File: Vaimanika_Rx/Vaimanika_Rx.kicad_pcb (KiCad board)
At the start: 4 copper layers, 18 x 25 mm, 54 parts, among them T1 0900PC16J0042001E, U1 LR1121IMLTRT, U2 RFX2401C, U3 SKY13373-460LF, U4 ESP32-C3FH4, U5 TLV75533PDQNR, U6 OW2EL89CENUXFMYLC-32M, U7 ANT3216LL00R2400A, U8 TS2306A 240GF MSM 9_C2976675, X1 CJ17-400001010B20

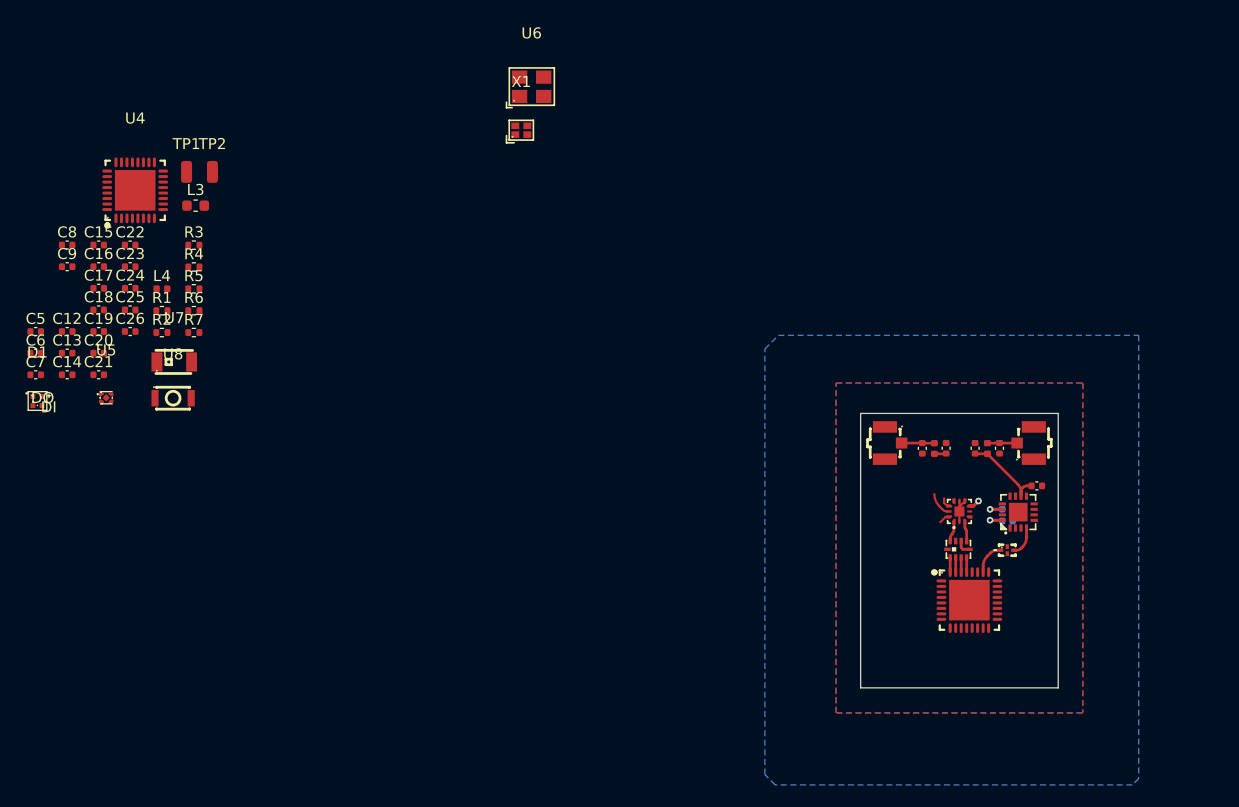
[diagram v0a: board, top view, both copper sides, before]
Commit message: 27-05-2026
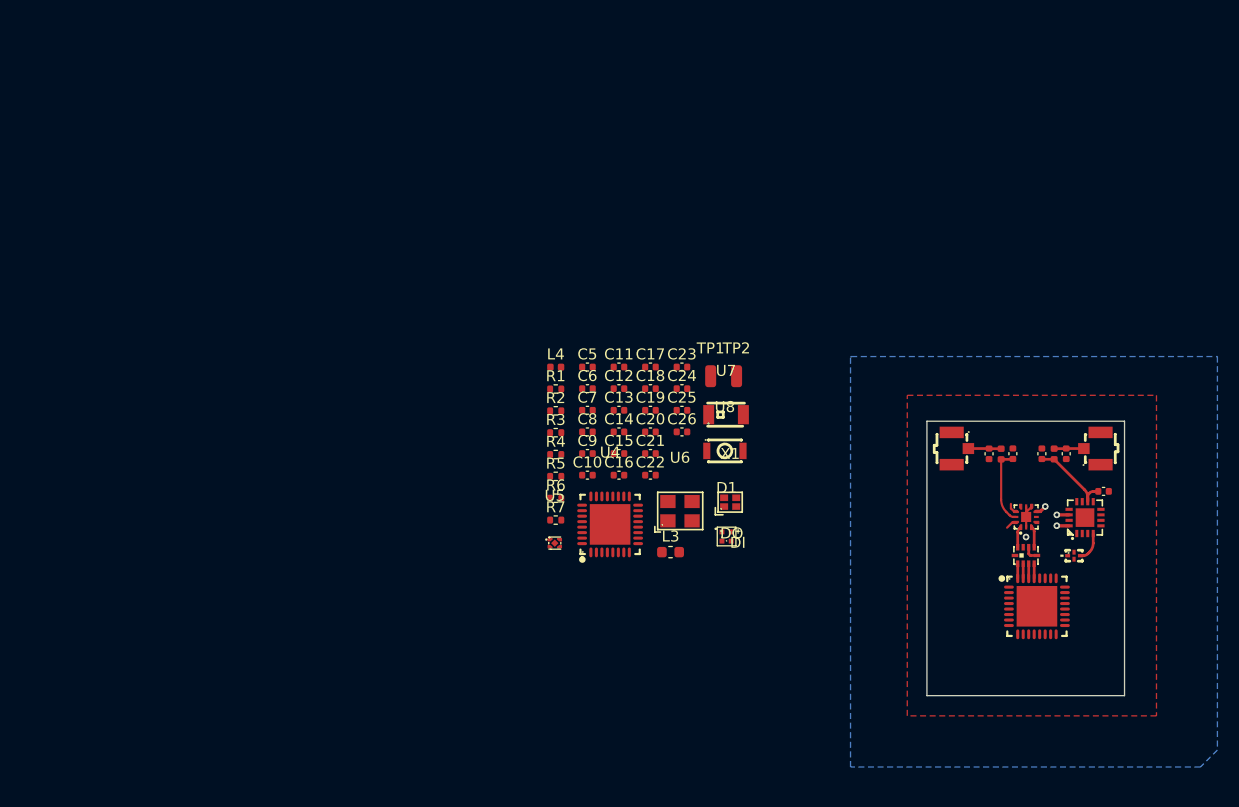
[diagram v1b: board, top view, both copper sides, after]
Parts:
- C10, C11: moved to F.Cu
- moved D1 64.0 mm to (124.7, 99.4)
- moved L3 53.6 mm to (119.6, 100.9)
- moved U4 52.9 mm to (114.1, 98.3)
- moved C22 51.8 mm to (117.8, 93.8)
- moved TP1 51.2 mm to (123.2, 84.8)
- moved TP2 51.2 mm to (125.6, 84.8)
- moved C23 51.1 mm to (120.6, 84.0)
- moved C24 51.1 mm to (120.6, 86.0)
- moved C25 51.1 mm to (120.6, 87.9)
- moved C26 51.1 mm to (120.6, 89.9)
- moved C15 51.1 mm to (114.9, 91.9)
- moved C16 51.1 mm to (114.9, 93.8)
- moved C17 50.8 mm to (117.8, 84.0)
- moved C18 50.8 mm to (117.8, 86.0)
- moved C19 50.8 mm to (117.8, 87.9)
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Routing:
- net Net-(U3-RFC): track 3.38 -> 7.03 mm
- net TXRX: track 2.98 -> 0.00 mm
- net GND: vias 0 -> 1
- removed copper zone on In2.Cu, net GND
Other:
- board text removed: "ELRS Reciver"
- board text removed: "Vaimanika Aerospace ELRS Receiver"
